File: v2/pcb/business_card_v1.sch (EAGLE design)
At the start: 69 parts, among them SW1 SPST_TACT-KMR2

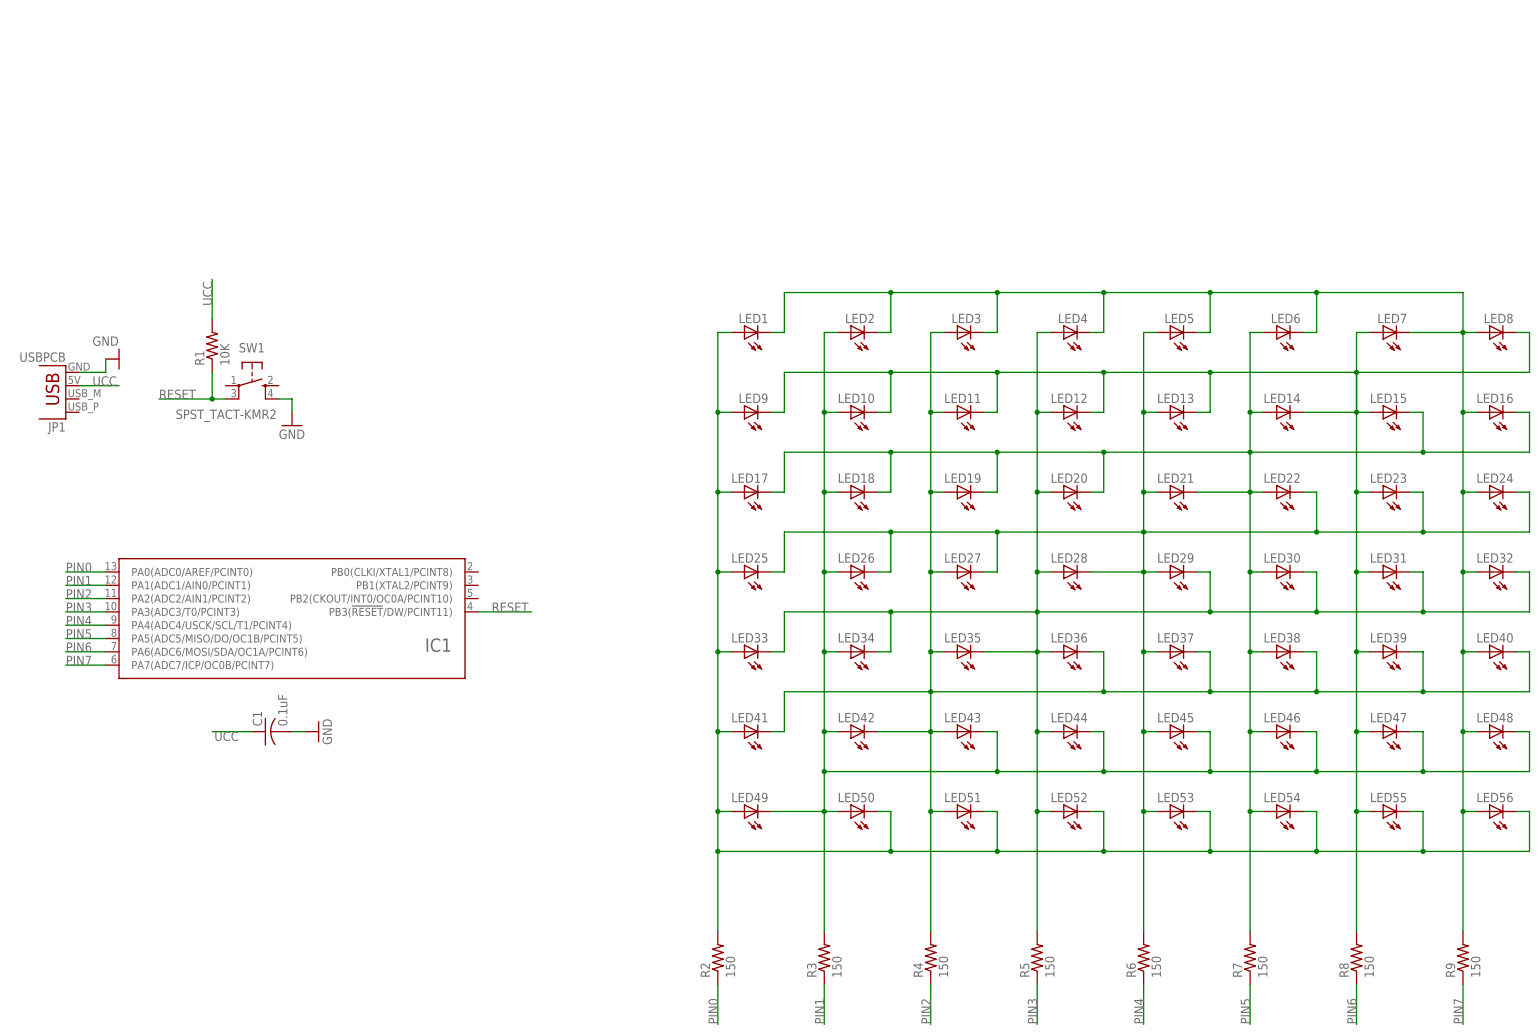
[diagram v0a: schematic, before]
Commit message: business card
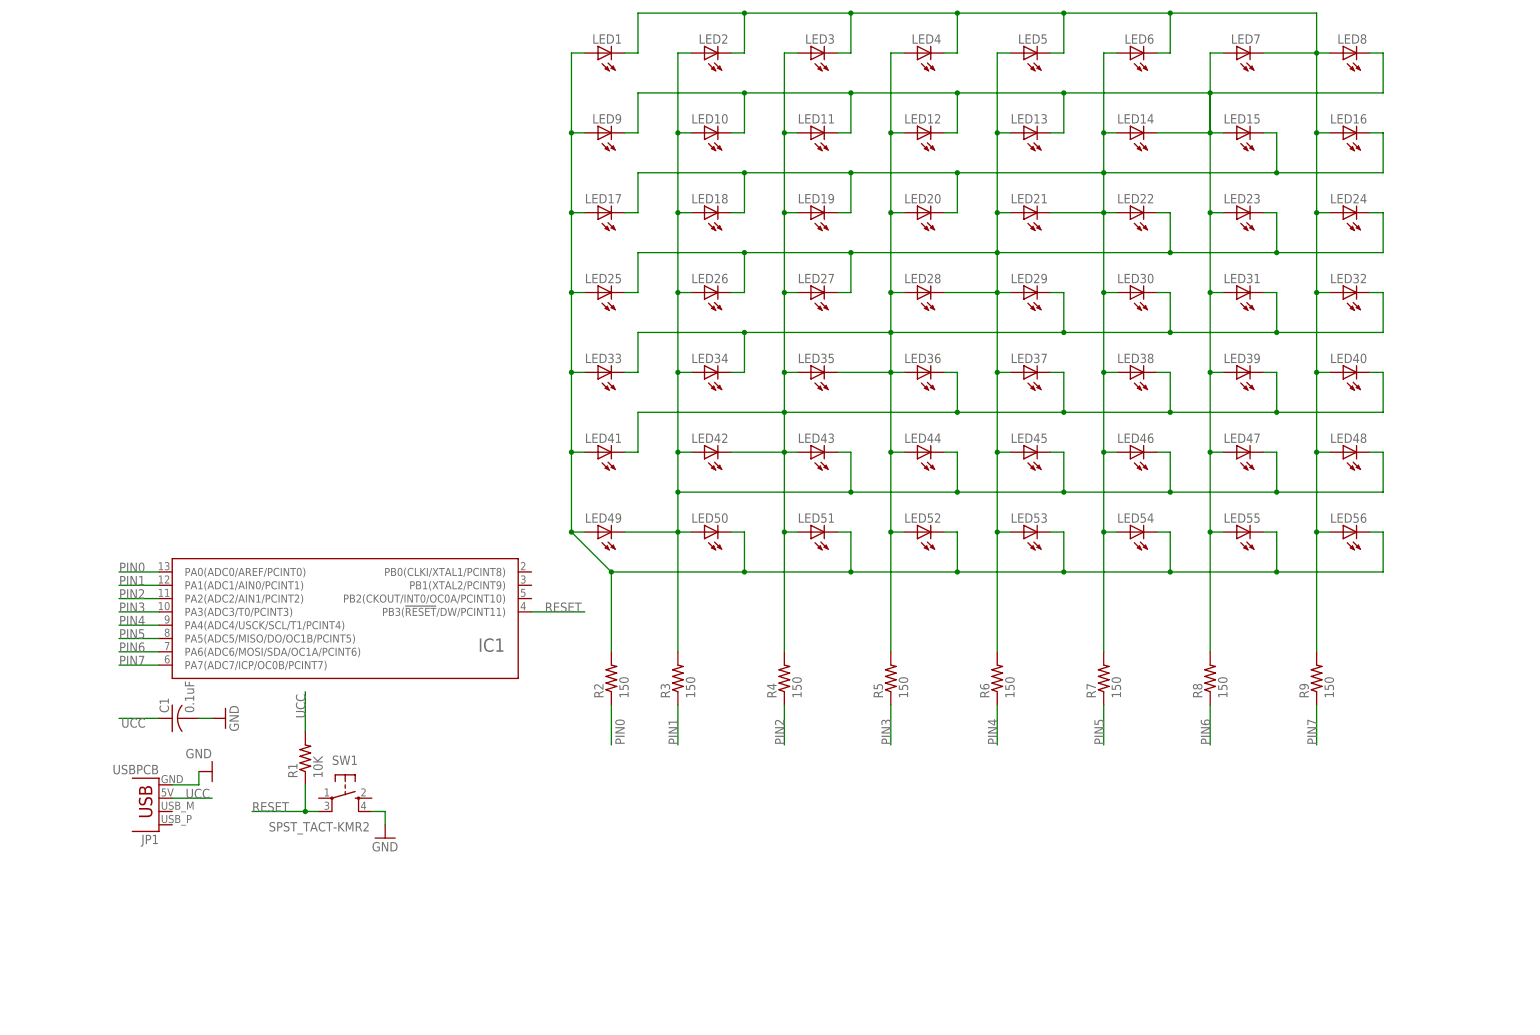
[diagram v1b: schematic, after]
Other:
- moved on the sheet: C1, IC1, JP1, LED1, LED10, LED11, LED12, LED13, LED14, LED15, LED16, LED17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
